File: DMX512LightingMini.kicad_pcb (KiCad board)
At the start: 2 copper layers, 45 x 30 mm, 36 parts, among them IC1 ADM4852ARZ, J1 Vin, J2 GND, J3 DATA+, J4 DATA-, Q1 2SC1815, Q2 Q_NMOS_GDS, Q3 2SC1815, Q4 Q_NMOS_GDS, Q5 2SC1815, Q6 Q_NMOS_GDS, U1 ATMEGA328PB-AU

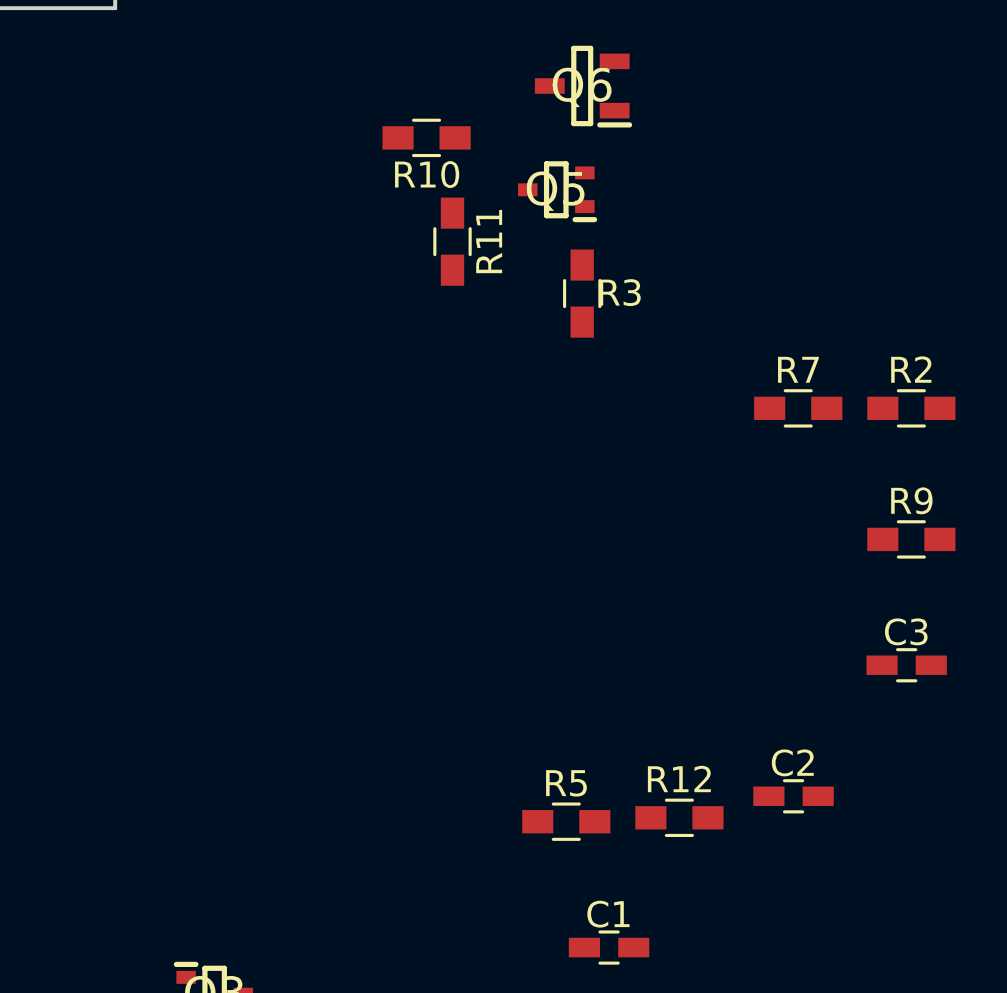
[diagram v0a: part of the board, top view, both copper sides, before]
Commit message: * AW作業中
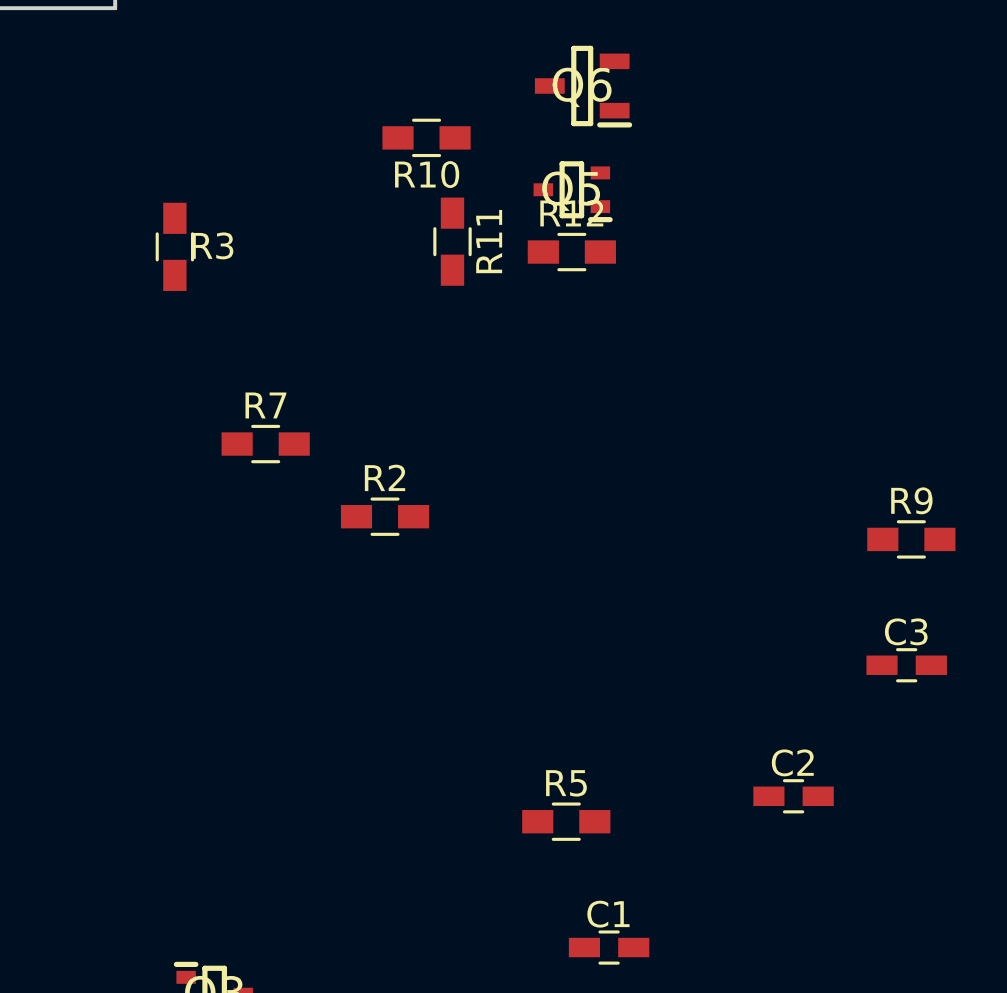
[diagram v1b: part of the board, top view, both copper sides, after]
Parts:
- moved R12 22.2 mm to (175.6, 122.4)
- moved R2 20.7 mm to (168.4, 132.6)
- moved R7 20.6 mm to (163.8, 129.8)
- moved R3 15.8 mm to (160.3, 122.2)
- moved Q5 0.60 mm to (175.6, 120.0)
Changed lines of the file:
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@@
   )
   (module SOT65P210X90-3N (layer F.Cu)
-    (at 175.03 120.03 180)
+    (at 175.63 120.03 180)
     (descr "UMT3_SOT-323 (SC70)")
     (tags Transistor)
     (attr smd)
-    (fp_text reference Q5 (at 0 0 180) (layer F.SilkS)
+    (fp_text reference Q5 (at 0 0 360) (layer F.SilkS)
       (effects (font (size 1.27 1.27) (thickness 0.254)))
     )
@@
     (tags Transistor)
     (attr smd)
-    (fp_text reference Q6 (at 0 0 180) (layer F.SilkS)
+    (fp_text reference Q6 (at 0 0 360) (layer F.SilkS)
       (effects (font (size 1.27 1.27) (thickness 0.254)))
     )
@@
   )
   (module Resistors_SMD:R_0603_HandSoldering (layer F.Cu)
-    (at 188.715001 128.455)
+    (at 168.43 132.63)
     (descr "Resistor SMD 0603, hand soldering")
     (tags "resistor 0603")
@@
   )
   (module Resistors_SMD:R_0603_HandSoldering (layer F.Cu)
-    (at 176.03 124.03 270)
+    (at 160.33 122.23 270)
     (descr "Resistor SMD 0603, hand soldering")
     (tags "resistor 0603")
@@
   )
   (module Resistors_SMD:R_0603_HandSoldering (layer F.Cu)
-    (at 184.355001 128.455)
+    (at 163.83 129.83)
     (descr "Resistor SMD 0603, hand soldering")
     (tags "resistor 0603")
@@
   )
   (module Resistors_SMD:R_0603_HandSoldering (layer F.Cu)
-    (at 179.775001 144.235)
-    (descr "Resistor SMD 0603, hand soldering")
-    (tags "resistor 0603")
+    (at 175.63 122.43)
+    (descr "Resistor SMD 0603, hand soldering")
+    (tags "resistor 0603")

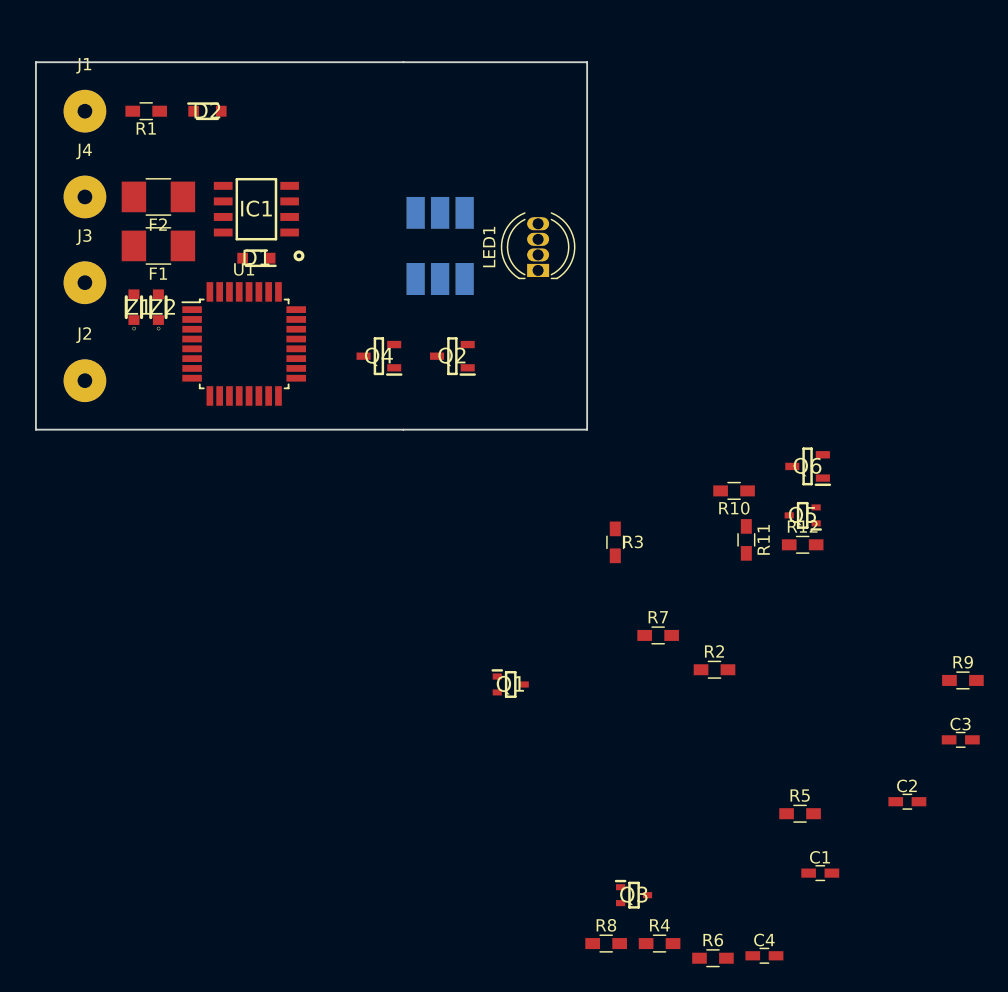
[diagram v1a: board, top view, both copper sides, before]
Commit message: * アートワーク作業中
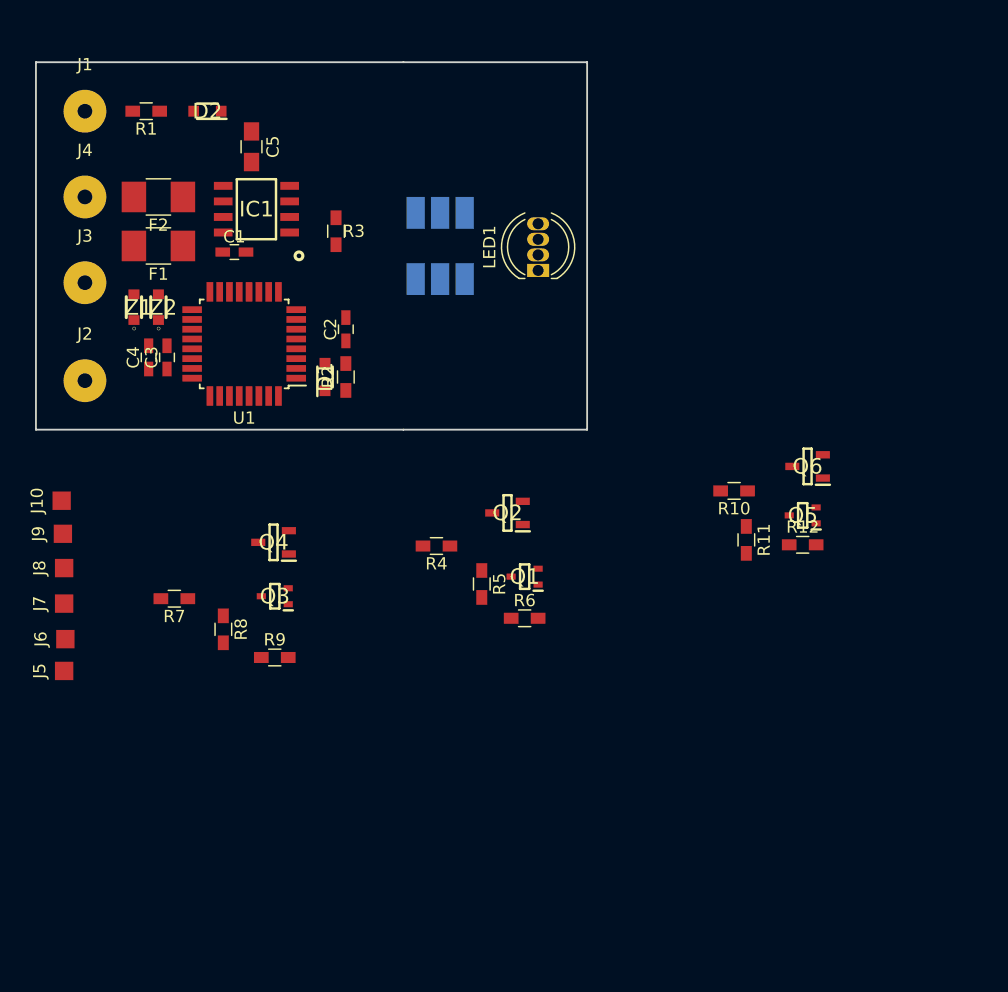
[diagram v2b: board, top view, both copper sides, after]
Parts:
- added C5: 10u, Capacitors_SMD:C_0805_HandSoldering, F.Cu at (130.6, 89.9)
- added J10: GND, Measurement_Points:Measurement_Point_Square-SMD-Pad_Small, F.Cu at (115.1, 118.8)
- added J5: RESET, Measurement_Points:Measurement_Point_Square-SMD-Pad_Small, F.Cu at (115.3, 132.7)
- added J6: MOSI, Measurement_Points:Measurement_Point_Square-SMD-Pad_Small, F.Cu at (115.4, 130.1)
- added J7: MISO, Measurement_Points:Measurement_Point_Square-SMD-Pad_Small, F.Cu at (115.3, 127.2)
- added J8: SCK, Measurement_Points:Measurement_Point_Square-SMD-Pad_Small, F.Cu at (115.3, 124.3)
- added J9: Vcc, Measurement_Points:Measurement_Point_Square-SMD-Pad_Small, F.Cu at (115.2, 121.5)
- moved C3 71.9 mm to (123.7, 107.1), turned to 90 degrees
- moved C4 70.1 mm to (122.2, 107.1), turned to 90 degrees
- moved C1 69.7 mm to (129.2, 98.5)
- moved C2 59.9 mm to (138.3, 104.8), turned to 90 degrees
- moved R9 56.2 mm to (132.5, 131.6)
- moved R8 40.4 mm to (128.3, 129.3), turned to 270 degrees
- moved R7 39.6 mm to (124.3, 126.8), turned to 180 degrees
- moved R2 38.4 mm to (138.3, 108.7), turned to 90 degrees
- moved Q3 38.2 mm to (132.5, 126.6), turned to 180 degrees
- moved R4 37.2 mm to (145.7, 122.5), turned to 180 degrees
- moved R3 34.1 mm to (137.5, 96.8)
- moved R5 32.0 mm to (149.4, 125.6), turned to 270 degrees
- moved R6 31.7 mm to (152.9, 128.4)
- moved Q4 17.5 mm to (132.4, 122.2)
- moved Q2 13.6 mm to (151.5, 119.8)
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
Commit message: * アートワーク完了    * 四角版
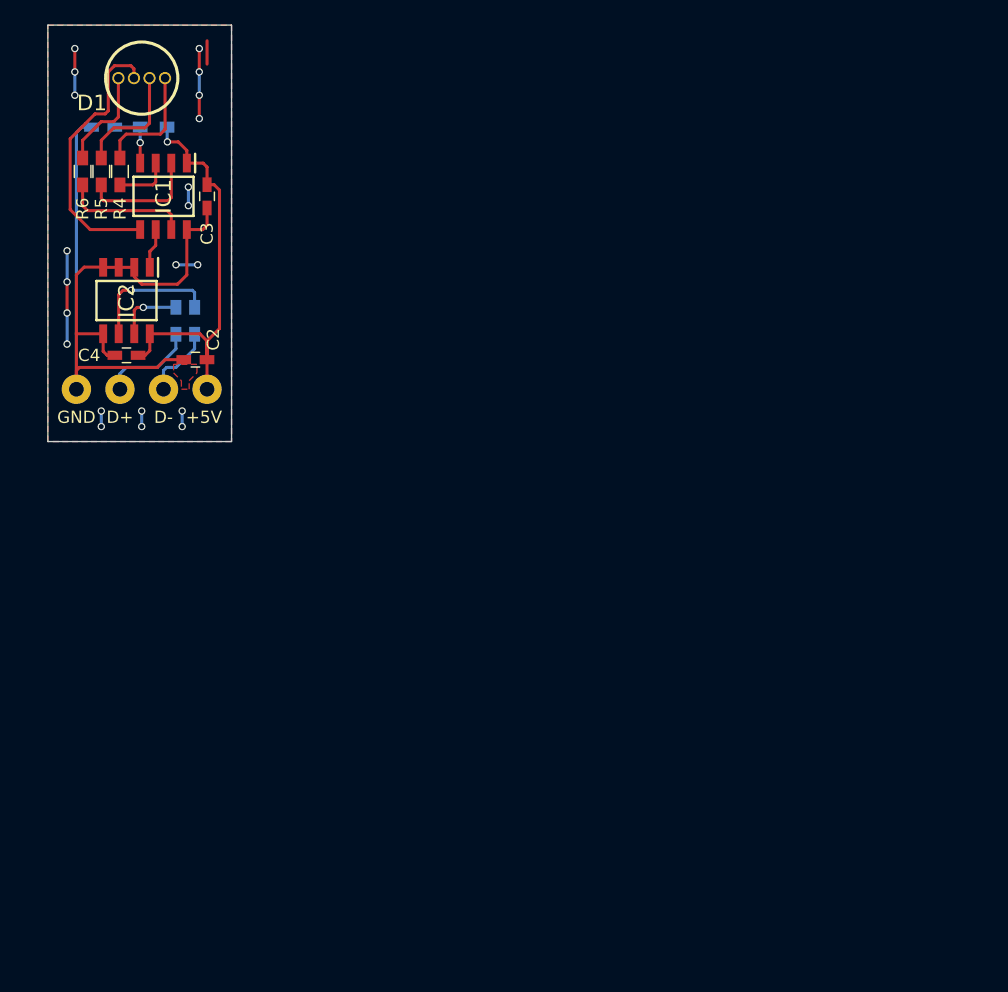
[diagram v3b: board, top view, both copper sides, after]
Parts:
- removed C5: 10u, Capacitors_SMD:C_0805_HandSoldering
- removed D2: 1SS355TE-17, SODFL2512X90N
- removed F1, F2: Polyfuse, Resistors_SMD:R_1210_HandSoldering
- removed J1: Vin, Wire_Pads:SolderWirePad_single_1-2mmDrill
- removed J10: GND, Measurement_Points:Measurement_Point_Square-SMD-Pad_Small
- removed J2: GND, Wire_Pads:SolderWirePad_single_1-2mmDrill
- removed J3: DATA+, Wire_Pads:SolderWirePad_single_1-2mmDrill
- removed J4: DATA-, Wire_Pads:SolderWirePad_single_1-2mmDrill
- removed J5: RESET, Measurement_Points:Measurement_Point_Square-SMD-Pad_Small
- removed J6: MOSI, Measurement_Points:Measurement_Point_Square-SMD-Pad_Small
- removed J7: MISO, Measurement_Points:Measurement_Point_Square-SMD-Pad_Small
- removed J8: SCK, Measurement_Points:Measurement_Point_Square-SMD-Pad_Small
- removed J9: Vcc, Measurement_Points:Measurement_Point_Square-SMD-Pad_Small
- removed LED1: LED_RGB_Anode_Pin3, LEDs:LED_D5.0mm-4
- removed LED2: SLC-F129CA-T1, SLC-F129CA-T1
- removed Q1, Q3, Q5: 2SC1815, SOT65P210X90-3N
- removed Q2, Q4, Q6: Q_NMOS_GDS, SOT95P280X100-3N
- removed R10, R11, R12, R7, R8, R9: R, Resistors_SMD:R_0603_HandSoldering
- removed U1: ATMEGA328PB-AU, Housings_QFP:TQFP-32_7x7mm_Pitch0.8mm
- removed Z1, Z2: UDZVTE-175.1B, UMD2_SOD-323F
- added +5V: +5V, Wire_Pads:SolderWirePad_single_1-2mmDrill, F.Cu at (127.0, 109.7)
- added D+: DATA+, Wire_Pads:SolderWirePad_single_1-2mmDrill, F.Cu at (119.9, 109.7)
- added D-: DATA-, Wire_Pads:SolderWirePad_single_1-2mmDrill, F.Cu at (123.4, 109.7)
- added GND: GND, Wire_Pads:SolderWirePad_single_1-2mmDrill, F.Cu at (116.3, 109.7)
- added IC2: ADM4852ARZ, SOIC127P600X175-8N, F.Cu at (120.4, 102.5)
- C1: moved to B.Cu
- C3: value 1u -> 0.1u
- D1: value 1SS355TE-17 -> L-154A4SURKQBDZGW; footprint SODFL2512X90N -> KNIGHTBRIGHT-1.27PITCH-4PIN
- IC1: value ADM4852ARZ -> PIC12F1840-I_SN
- R1: value R -> 10k; moved to B.Cu
- R2: value 1k -> 100; moved to B.Cu
- R3: value 10k -> 100; moved to B.Cu
- R4, R5, R6: value R -> 330
- moved R6 51.3 mm to (116.8, 91.9), turned to 90 degrees
- moved R5 45.8 mm to (118.4, 91.9)
- moved R4 40.0 mm to (119.9, 91.9), turned to 90 degrees
- moved D1 28.6 mm to (121.7, 84.3), turned to 0 degrees
- moved C1 14.8 mm to (118.5, 88.3), turned to 180 degrees
- moved R2 14.6 mm to (124.5, 104.1)
- moved R3 13.7 mm to (126.0, 104.1), turned to 90 degrees
- moved C3 13.6 mm to (127.0, 94.0), turned to 270 degrees
- moved C2 12.5 mm to (126.0, 107.3), turned to 180 degrees
- moved IC1 7.66 mm to (123.4, 94.0), turned to 270 degrees
- moved C4 1.82 mm to (120.4, 107.0), turned to 180 degrees
- moved R1 1.43 mm to (122.6, 88.3)
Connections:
- C1 pad 1: GND -> Net-(C1-Pad1)
- C1 pad 2: +5V -> GND
- C2 pad 1: Net-(C2-Pad1) -> +5V
- C3 pad 1: GND -> +5V
- C3 pad 2: +5V -> GND
- C4 pad 1: GND -> +5V
- C4 pad 2: +5V -> GND
- D1 pad 1: +5V -> Net-(D1-Pad1)
- D1 pad 2: Net-(C2-Pad1) -> Net-(D1-Pad2)
- IC1 pad 1: Net-(IC1-Pad1) -> +5V
- IC1 pad 3: Net-(IC1-Pad2) -> Net-(IC1-Pad3)
- IC1 pad 4: Net-(IC1-Pad4) -> Net-(C1-Pad1)
- IC1 pad 5: +5V -> Net-(D1-Pad2)
- IC1 pad 7: Net-(F1-Pad1) -> Net-(IC1-Pad7)
- R1 pad 1: Net-(D2-Pad2) -> +5V
- R1 pad 2: Net-(J1-Pad1) -> Net-(C1-Pad1)
- R2 pad 1: +5V -> Net-(R2-Pad1)
- R2 pad 2: Net-(C2-Pad1) -> DATA+
- R3 pad 1: Net-(IC1-Pad2) -> Net-(R3-Pad1)
- R3 pad 2: GND -> DATA-
- R4 pad 1: Net-(Q1-Pad2) -> Net-(IC1-Pad3)
- R4 pad 2: Net-(R4-Pad2) -> Net-(D1-Pad4)
- R5 pad 1: Net-(Q1-Pad2) -> Net-(D1-Pad3)
- R5 pad 2: GND -> Net-(IC1-Pad2)
- R6 pad 1: Net-(Q1-Pad3) -> Net-(IC1-Pad7)
- R6 pad 2: GND -> Net-(D1-Pad1)
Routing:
- net GND: track 0.00 -> 64.6 mm
- net +5V: track 0.00 -> 34.2 mm, vias 0 -> 1
- net (no net): track 0.00 -> 26.2 mm, vias 0 -> 21
- net Net-(D1-Pad2): track 0.00 -> 22.6 mm
- net DATA-: track 0.00 -> 10.8 mm, vias 0 -> 1
- net Net-(IC1-Pad7): track 0.00 -> 10.5 mm
- net Net-(IC1-Pad2): track 0.00 -> 9.82 mm
- net Net-(D1-Pad4): track 0.00 -> 9.68 mm
- net Net-(D1-Pad3): track 0.00 -> 9.64 mm
- net Net-(D1-Pad1): track 0.00 -> 8.33 mm
- net Net-(R2-Pad1): track 0.00 -> 7.87 mm
- net Net-(R3-Pad1): track 0.00 -> 5.99 mm
- net DATA+: track 0.00 -> 5.43 mm, vias 0 -> 1
- net Net-(C1-Pad1): track 0.00 -> 5.01 mm, vias 0 -> 1
- net Net-(IC1-Pad3): track 0.00 -> 4.56 mm
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- added copper zone on B.Cu, net GND
- added copper zone on F.Cu, net GND
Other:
- board size 45 x 30 mm -> 15 x 34 mm
- rule pad_to_mask_clearance: 0.2 -> 0
